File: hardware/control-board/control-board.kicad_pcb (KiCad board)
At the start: 2 copper layers, 39.5 x 106.5 mm, 28 parts, among them J1 JACK_2P, J12 JACK_2P, J14 Top Left(M), J16 Top Right (M), J18 Bottom Left(M), J2 JACK_2P, J20 Bottom Right(M), J3 JACK_2P, J4 JACK_2P, J5 JACK_2P, J6 JACK_2P, J7 JACK_2P, J8 JACK_2P

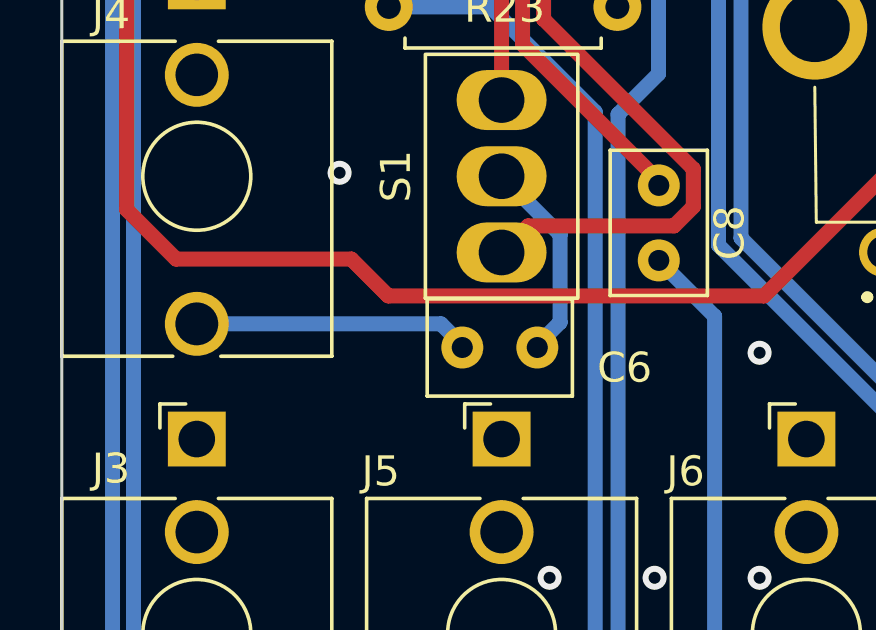
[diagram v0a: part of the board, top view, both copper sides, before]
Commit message: chore: restructure project
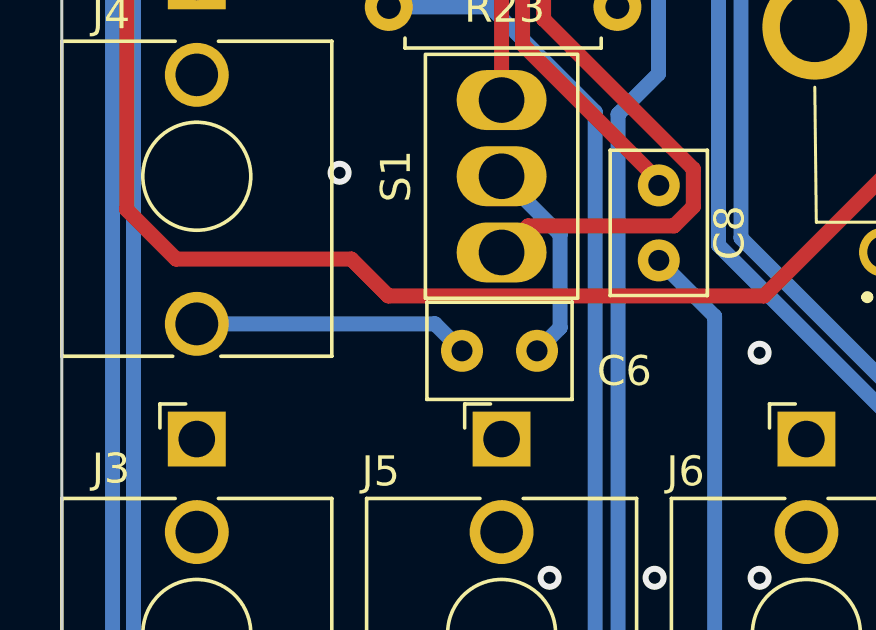
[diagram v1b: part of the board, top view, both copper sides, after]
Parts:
- RV3, RV4, RV5: footprint cem-3340:Alpha Potentiometer -> Eurorack Common:Alpha Potentiometer
- S1: footprint cem-3340:Sub-Miniature SPDT -> Eurorack Common:Sub-Miniature SPDT
- moved C6 0.11 mm to (28.6, 90.4)
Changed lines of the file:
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@@
 		)
 		(embedded_fonts no)
-		(model "${KIPRJMOD}/../libs/3D/Thonkicon.step"
+		(model "${KIPRJMOD}/../shared/3dmodels/Thonkicon.step"
 			(offset
 				(xyz 0 -7 0)
@@
 		)
 		(embedded_fonts no)
-		(model "${KIPRJMOD}/../libs/3D/Thonkicon.step"
+		(model "${KIPRJMOD}/../shared/3dmodels/Thonkicon.step"
 			(offset
 				(xyz 0 -7 0)
@@
 		)
 	)
-	(footprint "cem-3340:Sub-Miniature SPDT"
+	(footprint "Eurorack Common:Sub-Miniature SPDT"
 		(layer "F.Cu")
 		(at 29.9 84.616 90)
@@
 			)
 		)
-		(property "Datasheet" "~"
+		(property "Datasheet" ""
 			(at 0 0 90)
 			(layer "F.Fab")
@@
 			)
 		)
-		(property "Description" "Switch, single pole double throw"
+		(property "Description" ""
 			(at 0 0 90)
 			(layer "F.Fab")
@@
 		)
 		(embedded_fonts no)
-		(model "${KIPRJMOD}/../libs/3D/200-MSP-1-T3-B1-M2-PE-rev2.step"
+		(model "${KIPRJMOD}/../shared/3dmodels/Subminiture-SPDT.step"
 			(offset
 				(xyz 0 0 0)
@@
 		)
 	)
-	(footprint "cem-3340:Alpha Potentiometer"
+	(footprint "Eurorack Common:Alpha Potentiometer"
 		(layer "F.Cu")
 		(at 22.315 71.871)
@@
 			)
 		)
-		(property "Datasheet" "~"
+		(property "Datasheet" ""
 			(at 0 0 0)
 			(layer "F.Fab")
@@
 			)
 		)
-		(property "Description" "Potentiometer"
+		(property "Description" ""
 			(at 0 0 0)
 			(layer "F.Fab")
@@
 		)
 		(embedded_fonts no)
-		(model "${KIPRJMOD}/../libs/3D/ALPHA-RD901F-40.step"
+		(model "${KIPRJMOD}/../shared/3dmodels/Alpha-Pot.step"
 			(offset
-				(xyz 2.5 7 7)
+				(xyz 2.5 7.5 7)
 			)
 			(scale
@@
 		)
 		(embedded_fonts no)
-		(model "${KIPRJMOD}/../libs/3D/Thonkicon.step"
+		(model "${KIPRJMOD}/../shared/3dmodels/Thonkicon.step"
 			(offset
 				(xyz 0 -7 0)
@@
 		)
 		(embedded_fonts no)
-		(model "${KIPRJMOD}/../libs/3D/Thonkicon.step"
+		(model "${KIPRJMOD}/../shared/3dmodels/Thonkicon.step"
 			(offset
 				(xyz 0 -7 0)
@@
 		)
 	)
-	(footprint "cem-3340:Alpha Potentiometer"
+	(footprint "Eurorack Common:Alpha Potentiometer"
 		(layer "F.Cu")
 		(at 32.465 40.896)
@@
 			)
 		)
-		(property "Datasheet" "~"
+		(property "Datasheet" ""
 			(at 0 0 0)
 			(layer "F.Fab")
@@
 			)
 		)
-		(property "Description" "Potentiometer"
+		(property "Description" ""
 			(at 0 0 0)
 			(layer "F.Fab")
@@
 		)
 		(embedded_fonts no)
-		(model "${KIPRJMOD}/../libs/3D/ALPHA-RD901F-40.step"
+		(model "${KIPRJMOD}/../shared/3dmodels/Alpha-Pot.step"
 			(offset
-				(xyz 2.5 7 7)
+				(xyz 2.5 7.5 7)
 			)
 			(scale
@@
 		)
 	)
-	(footprint "cem-3340:Alpha Potentiometer"
+	(footprint "Eurorack Common:Alpha Potentiometer"
 		(layer "F.Cu")
 		(at 42.64 87.146)
@@
 			)
 		)
-		(property "Datasheet" "~"
+		(property "Datasheet" ""
 			(at 0 0 0)
 			(layer "F.Fab")
@@
 			)
 		)
-		(property "Description" "Potentiometer"
+		(property "Description" ""
 			(at 0 0 0)
 			(layer "F.Fab")
@@
 		)
 		(embedded_fonts no)
-		(model "${KIPRJMOD}/../libs/3D/ALPHA-RD901F-40.step"
+		(model "${KIPRJMOD}/../shared/3dmodels/Alpha-Pot.step"
 			(offset
-				(xyz 2.5 7.5 7.5)
+				(xyz 2.5 7.5 7)
 			)
 			(scale
@@
 		)
 		(embedded_fonts no)
-		(model "${KIPRJMOD}/../libs/3D/Thonkicon.step"
+		(model "${KIPRJMOD}/../shared/3dmodels/Thonkicon.step"
 			(offset
 				(xyz 0 -7 0)
@@
 		)
 		(embedded_fonts no)
-		(model "${KIPRJMOD}/../libs/3D/Thonkicon.step"
+		(model "${KIPRJMOD}/../shared/3dmodels/Thonkicon.step"
 			(offset
 				(xyz 0 -7 0)
@@
 		)
 		(embedded_fonts no)
-		(model "${KIPRJMOD}/../libs/3D/Thonkicon.step"
+		(model "${KIPRJMOD}/../shared/3dmodels/Thonkicon.step"
 			(offset
 				(xyz 0 -7 0)
@@
 	(footprint "Capacitor_THT:C_Rect_L4.6mm_W3.0mm_P2.50mm_MKS02_FKP02"
 		(layer "F.Cu")
-		(at 28.59 90.324)
+		(at 28.580556 90.434755)
 		(descr "C, Rect series, Radial, pin pitch=2.50mm, length*width=4.6*3.0mm^2, Capacitor, http://www.wima.de/DE/WIMA_MKS_02.pdf")
 		(tags "C Rect series Radial pin pitch 2.50mm length 4.6mm width 3.0mm Capacitor")
@@
 		)
 		(embedded_fonts no)
-		(model "${KIPRJMOD}/../libs/3D/Thonkicon.step"
+		(model "${KIPRJMOD}/../shared/3dmodels/Thonkicon.step"
 			(offset
 				(xyz 0 -7 0)
@@
 		)
 		(embedded_fonts no)
-		(model "${KIPRJMOD}/../libs/3D/Thonkicon.step"
+		(model "${KIPRJMOD}/../shared/3dmodels/Thonkicon.step"
 			(offset
 				(xyz 0 -7 0)
@@
 	)
 	(segment
-		(start 29.90993 84.616)
-		(end 31.84952 86.55559)
+		(start 31.84952 86.55559)
+		(end 31.84952 89.665791)
 		(width 0.5)
 		(layer "B.Cu")
@@
 	)
 	(segment
-		(start 31.84952 86.55559)
-		(end 31.84952 89.48648)
+		(start 29.90993 84.616)
+		(end 31.84952 86.55559)
 		(width 0.5)
 		(layer "B.Cu")
@@
 	)
 	(segment
-		(start 31.84952 89.48648)
-		(end 31.09 90.246)
+		(start 29.9 84.616)
+		(end 29.90993 84.616)
 		(width 0.5)
 		(layer "B.Cu")
@@
 	)
 	(segment
-		(start 29.9 84.616)
-		(end 29.90993 84.616)
+		(start 31.84952 89.665791)
+		(end 31.080556 90.434755)
 		(width 0.5)
 		(layer "B.Cu")
@@
 	)
 	(segment
-		(start 27.88 89.536)
-		(end 28.59 90.246)
+		(start 27.681801 89.536)
+		(end 28.580556 90.434755)
 		(width 0.5)
 		(layer "B.Cu")
@@
 	(segment
 		(start 19.74 89.536)
-		(end 27.88 89.536)
+		(end 27.681801 89.536)
 		(width 0.5)
 		(layer "B.Cu")
